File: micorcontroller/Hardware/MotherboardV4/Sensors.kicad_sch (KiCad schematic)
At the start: 53 parts

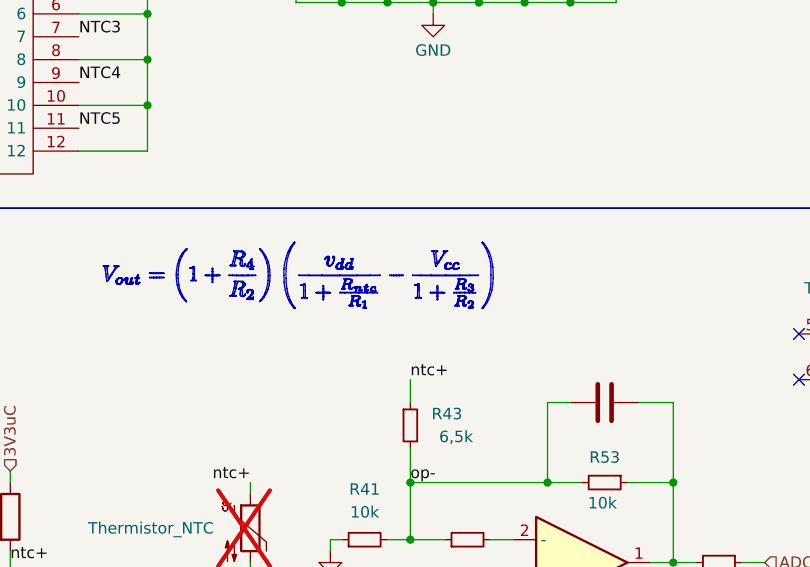
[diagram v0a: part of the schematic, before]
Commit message: startup message
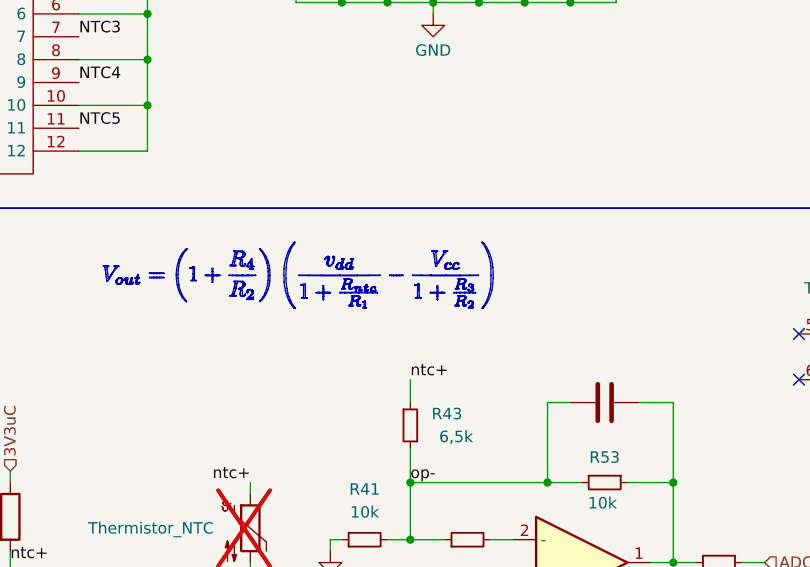
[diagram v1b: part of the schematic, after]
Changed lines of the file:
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@@
 	)
 	(arc
-		(start 81.2439 132.6404)
-		(mid 81.244 132.6596)
-		(end 81.2369 132.6487)
+		(start 81.2369 132.6487)
+		(mid 81.2388 132.6431)
+		(end 81.2439 132.6404)
 		(stroke
 			(width 0.08)
@@
 	)
 	(arc
-		(start 95.35 138.0726)
-		(mid 95.3708 138.0738)
-		(end 95.3605 138.0844)
+		(start 95.3605 138.0844)
+		(mid 95.3514 138.0815)
+		(end 95.35 138.0726)
 		(stroke
 			(width 0.08)
@@
 	)
 	(arc
-		(start 85.0546 136.1217)
-		(mid 85.0391 136.1162)
-		(end 85.0477 136.107)
+		(start 85.0477 136.107)
+		(mid 85.0601 136.1115)
+		(end 85.0546 136.1217)
 		(stroke
 			(width 0.08)
@@
 	)
 	(arc
-		(start 82.4029 136.7281)
-		(mid 82.4004 136.7249)
-		(end 82.4032 136.7206)
+		(start 82.4032 136.7206)
+		(mid 82.4025 136.7221)
+		(end 82.4029 136.7281)
 		(stroke
 			(width 0.08)
@@
 	)
 	(arc
-		(start 94.281 135.9581)
-		(mid 94.2805 135.9581)
-		(end 94.28 135.9518)
+		(start 94.28 135.9518)
+		(mid 94.2839 135.9543)
+		(end 94.281 135.9581)
 		(stroke
 			(width 0.08)

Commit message: added uplink
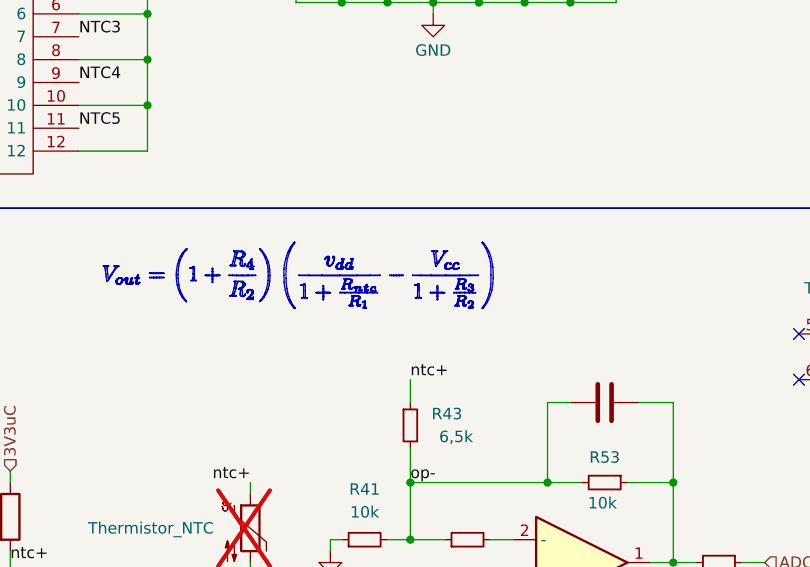
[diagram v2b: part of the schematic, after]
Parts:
- BAR0: symbol SamacSys_Parts:MS561101BA03-50 -> SymbolsBalloonv4:MS561101BA03-50
- C40, C41, C42, C43, C44, C45: symbol Device:C -> SymbolsBalloonv4:C
- F0: symbol Device:Fuse_Small -> SymbolsBalloonv4:Fuse_Small
- JP3, JP4, JP5, JP6, JP7, JP8: symbol Jumper:SolderJumper_2_Open -> SymbolsBalloonv4:SolderJumper_2_Open
- JP9, JPVOX0, JPVOX1: symbol Jumper:SolderJumper_3_Open -> SymbolsBalloonv4:SolderJumper_3_Open
- LED1: symbol Device:LED_ARBG -> SymbolsBalloonv4:LED_ARBG
- MUX0: symbol SamacSys_Parts:TMUX1108PWR -> SymbolsBalloonv4:TMUX1108PWR
- NTCs0: symbol SamacSys_Parts:502352-1210 -> SymbolsBalloonv4:502352-1210
- OP1: symbol Device:Opamp_Dual -> SymbolsBalloonv4:Opamp_Dual
- Ox0, RS-0: symbol SamacSys_Parts:502352-0400 -> SymbolsBalloonv4:502352-0400
- R37: symbol Device:R -> SymbolsBalloonv4:R
- R38, R39, R40, R41, R42, R43, R44, R45, R46, R47, R48, R49, R50, R51, R52, R53, R54, R55, R56, R57, R58, R59, R60, R61, R62: symbol Device:R_Small -> SymbolsBalloonv4:R_Small
- RS0: symbol SamacSys_Parts:MAX3485AEASA+T -> SymbolsBalloonv4:MAX3485AEASA+T
- RT0, TH0: symbol Device:Thermistor_NTC -> SymbolsBalloonv4:Thermistor_NTC
- Vref1: symbol Device:D_Zener -> SymbolsBalloonv4:D_Zener
